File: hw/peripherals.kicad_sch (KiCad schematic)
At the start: 1 part, among them Q2 RU1J002YN

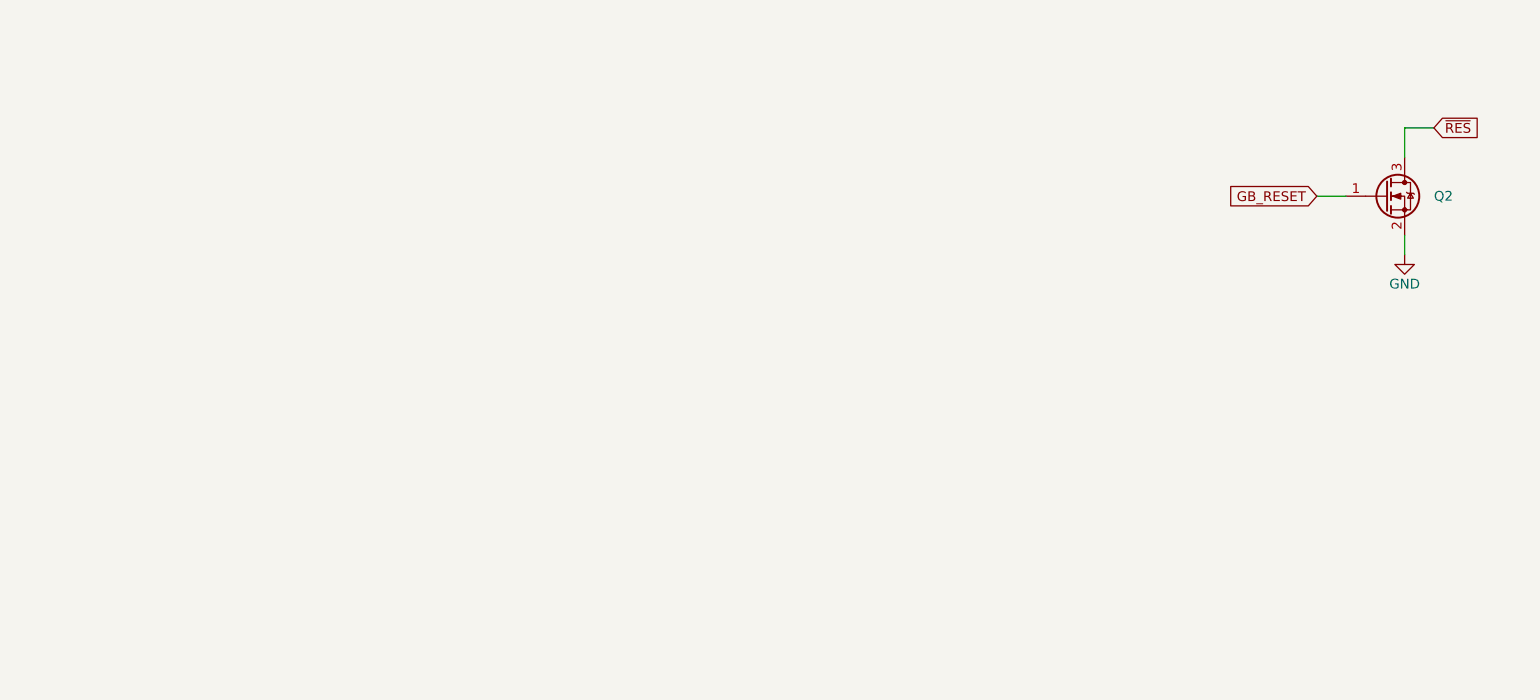
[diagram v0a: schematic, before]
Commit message: hw: complete 2-layer PCB
Signed-off-by: Mahyar Koshkouei <mk@deltabeard.com>
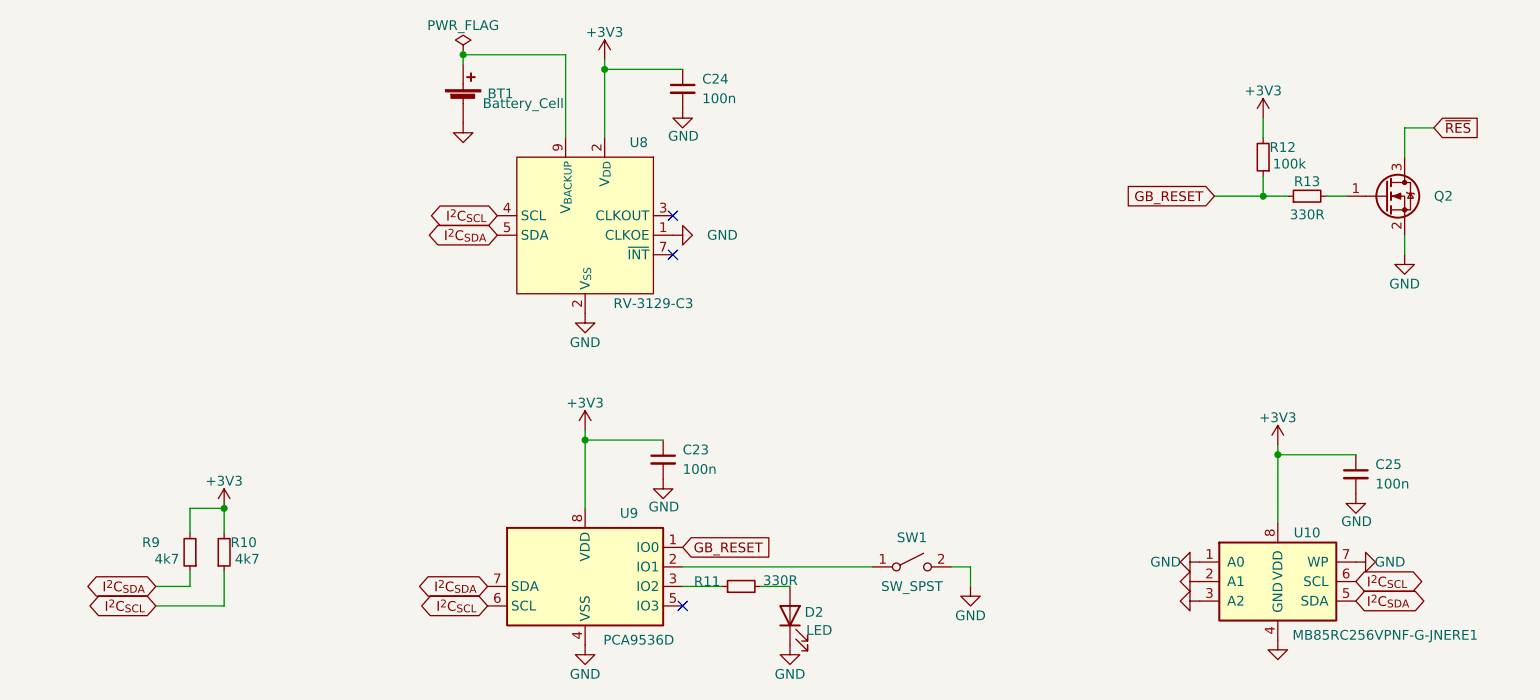
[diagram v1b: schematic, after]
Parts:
- added BT1: Battery_Cell, Project_Specific:BatteryHolder_Seiko_MS621FE, symbol Device:Battery_Cell
- added C23, C24, C25: 100n, Capacitor_SMD:C_0402_1005Metric, symbol Device:C_Small
- added D2: LED, LED_SMD:LED_0603_1608Metric, symbol Device:LED
- added R10, R9: 4k7, Resistor_SMD:R_0402_1005Metric, symbol Device:R_Small
- added R11, R13: 330R, Resistor_SMD:R_0603_1608Metric, symbol Device:R_Small
- added R12: 100k, Resistor_SMD:R_0603_1608Metric, symbol Device:R_Small
- added SW1: SW_SPST, Project_Specific:Push_Button-Horizontal-TC-1109DE-C-J, symbol Switch:SW_SPST
- added U10: MB85RC256VPNF-G-JNERE1, Package_SO:SOIC-8_3.9x4.9mm_P1.27mm, symbol Project_specific:MB85RC256V
- added U8: RV-3129-C3, Project_Specific:SOIC-10_RV-3129-C3, symbol Project_specific:RV-3129-C3
- added U9: PCA9536D, Package_SO:SOIC-8_3.9x4.9mm_P1.27mm, symbol Interface_Expansion:PCA9536D
- Q2: value RU1J002YN -> N-Channel; footprint Package_TO_SOT_SMD:SOT-323_SC-70 -> Package_TO_SOT_SMD:SOT-23; LCSC (none) -> C8545; MFr RU1J002YN -> 2N7002
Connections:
- net GB_RESET: now also R12.1, R13.1, U9.1 (IO0); no longer Q2.1 (G)
- net GND: now also BT1.2 (-), C23.2, C24.2, C25.2, D2.1 (K), SW1.2 (B), U10.1 (A0), U10.2 (A1), U10.3 (A2), U10.4 (GND), U10.7 (WP), U8.1 (CLKOE), U8.2 (V_{SS}), U9.4 (VSS)
- new net: BT1.1 (+), U8.9 (V_{BACKUP})
- new net: SW1.1 (A), U9.2 (IO1)
- new net: R11.1, U9.3 (IO2)
- new net: D2.2 (A), R11.2
- new net: Q2.1 (G), R13.2
- new net +3V3: C23.1, C24.1, C25.1, R10.2, R12.2, R9.2, U10.8 (VDD), U8.2 (V_{SS}), U9.8 (VDD)
- new net I^{2}C_{SCL}: R10.1, U10.6 (SCL), U8.4 (SCL), U9.6 (SCL)
- new net I^{2}C_{SDA}: R9.1, U10.5 (SDA), U8.5 (SDA), U9.7 (SDA)
- no-connect marks 0 -> 3
